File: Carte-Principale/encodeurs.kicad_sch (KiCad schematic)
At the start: 0 parts

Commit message: Moteurs + Encodeurs
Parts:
- added J3: Encodeur_G, symbol Connector:Conn_01x08_Pin
- added J4: Encodeur_D, symbol Connector:Conn_01x08_Pin
- added R1, R2, R3, R4: 100, symbol Device:R_Small
- added U6: AM26LV32xD, Package_SO:SOIC-16_3.9x9.9mm_P1.27mm, symbol Interface:AM26LV32xD
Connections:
- new net +3.3V: U6.16 (VDD), U6.4 (G)
- new net +5V: J3.1 (Pin_1), J4.1 (Pin_1)
- new net A+_DROITE: J4.6 (Pin_6), R4.2, U6.2 (1A)
- new net A+_GAUCHE: J3.6 (Pin_6), R2.2, U6.10 (3A)
- new net A-_DROITE: J4.7 (Pin_7), R4.1, U6.1 (1B)
- new net A-_GAUCHE: J3.7 (Pin_7), R2.1, U6.9 (3B)
- new net A_DROITE: U6.3 (1Y)
- new net A_GAUCHE: U6.11 (3Y)
- new net B+_DROITE: J4.5 (Pin_5), R3.2, U6.6 (2A)
- new net B+_GAUCHE: J3.5 (Pin_5), R1.2, U6.14 (4A)
- new net B-_DROITE: J4.4 (Pin_4), R3.1, U6.7 (2B)
- new net B-_GAUCHE: J3.4 (Pin_4), R1.1, U6.15 (4B)
- new net B_DROITE: U6.5 (2Y)
- new net B_GAUCHE: U6.13 (4Y)
- new net GND: J3.8 (Pin_8), J4.8 (Pin_8), U6.12 (~{G}), U6.8 (GND)
- new net Z+_DROITE: J4.2 (Pin_2)
- new net Z+_GAUCHE: J3.2 (Pin_2)
- new net Z-_DROITE: J4.3 (Pin_3)
- new net Z-_GAUCHE: J3.3 (Pin_3)
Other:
- note added: "Bien mettre dans le bon sens dans le PCB"

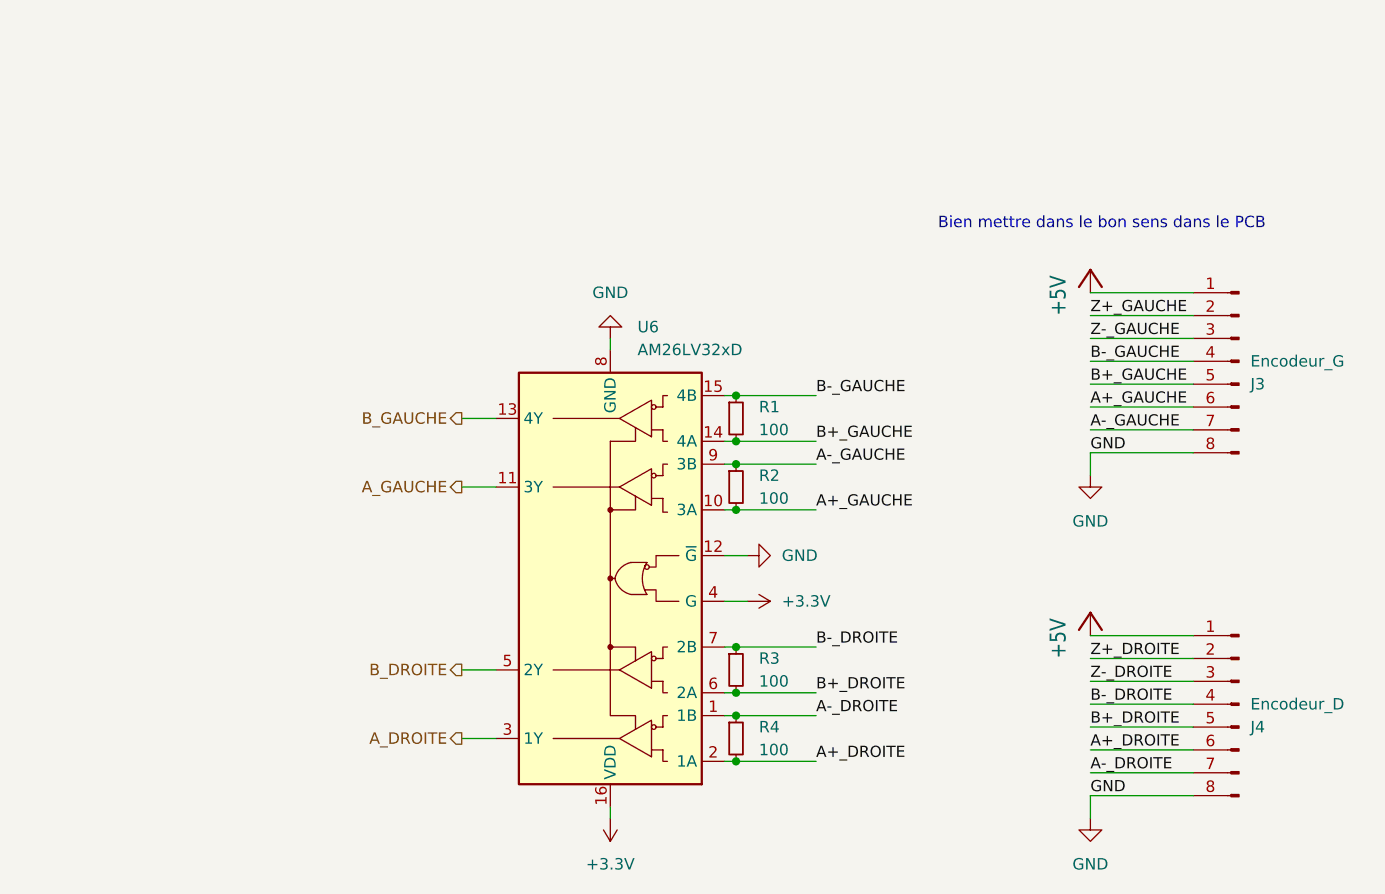
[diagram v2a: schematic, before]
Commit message: wiring
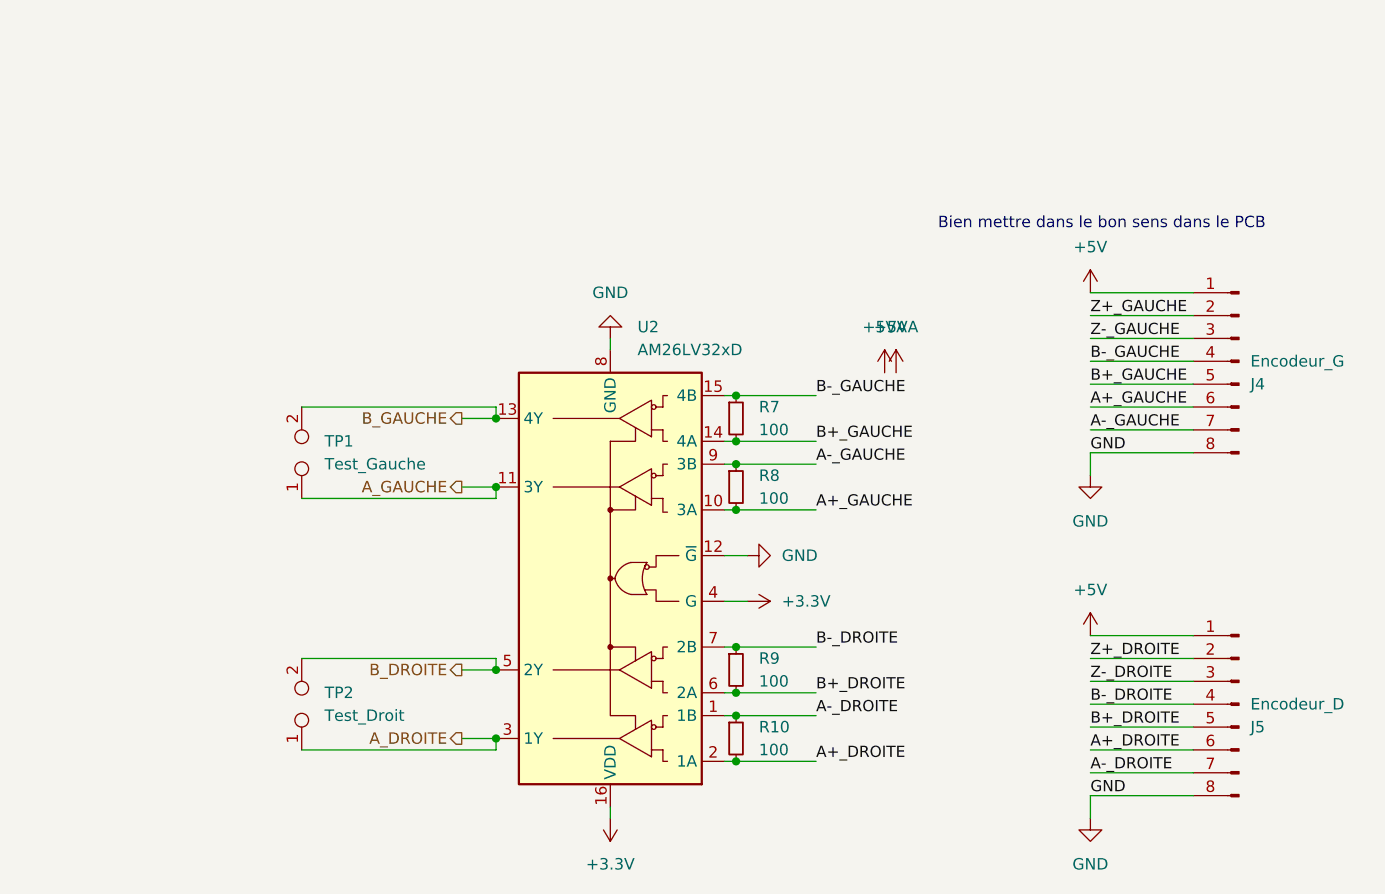
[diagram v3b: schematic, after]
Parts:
- added TP1: Test_Gauche, TestPoint:TestPoint_2Pads_Pitch2.54mm_Drill0.8mm, symbol Connector:TestPoint_2Pole
- added TP2: Test_Droit, TestPoint:TestPoint_2Pads_Pitch2.54mm_Drill0.8mm, symbol Connector:TestPoint_2Pole
- J4: renamed from J3; footprint (none) -> Connector_PinHeader_2.54mm:PinHeader_1x08_P2.54mm_Vertical
- J5: renamed from J4; footprint (none) -> Connector_PinHeader_2.54mm:PinHeader_1x08_P2.54mm_Vertical
- R10: renamed from R4; footprint (none) -> Resistor_THT:R_Axial_DIN0207_L6.3mm_D2.5mm_P10.16mm_Horizontal
- R7: renamed from R1; footprint (none) -> Resistor_THT:R_Axial_DIN0207_L6.3mm_D2.5mm_P10.16mm_Horizontal
- R8: renamed from R2; footprint (none) -> Resistor_THT:R_Axial_DIN0207_L6.3mm_D2.5mm_P10.16mm_Horizontal
- R9: renamed from R3; footprint (none) -> Resistor_THT:R_Axial_DIN0207_L6.3mm_D2.5mm_P10.16mm_Horizontal
- renumbered U6 to U2
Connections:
- net A_DROITE: now also TP2.1
- net A_GAUCHE: now also TP1.1
- net B_DROITE: now also TP2.2
- net B_GAUCHE: now also TP1.2

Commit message: Schéma vérifié
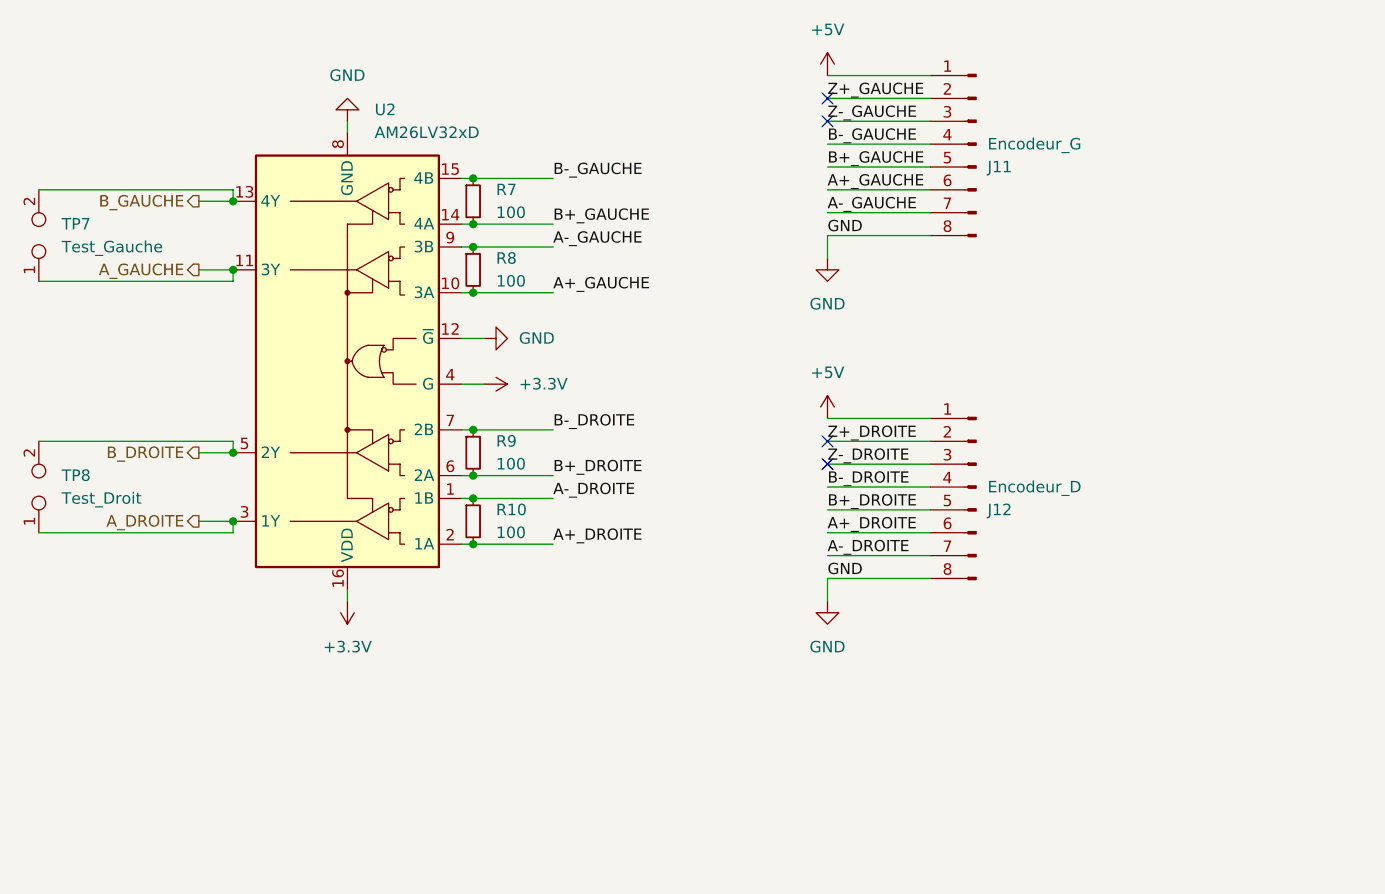
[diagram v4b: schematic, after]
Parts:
- renumbered J4 to J11, J5 to J12, TP1 to TP7, TP2 to TP8
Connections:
- no-connect marks 0 -> 4
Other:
- note removed: "Bien mettre dans le bon sens dans le PCB"
- company: (none) -> CRINSA
- title: (none) -> Carte Principale
- moved on the sheet: J11, J12, R10, R7, R8, R9, TP7, TP8, U2

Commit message: Avancée PCB
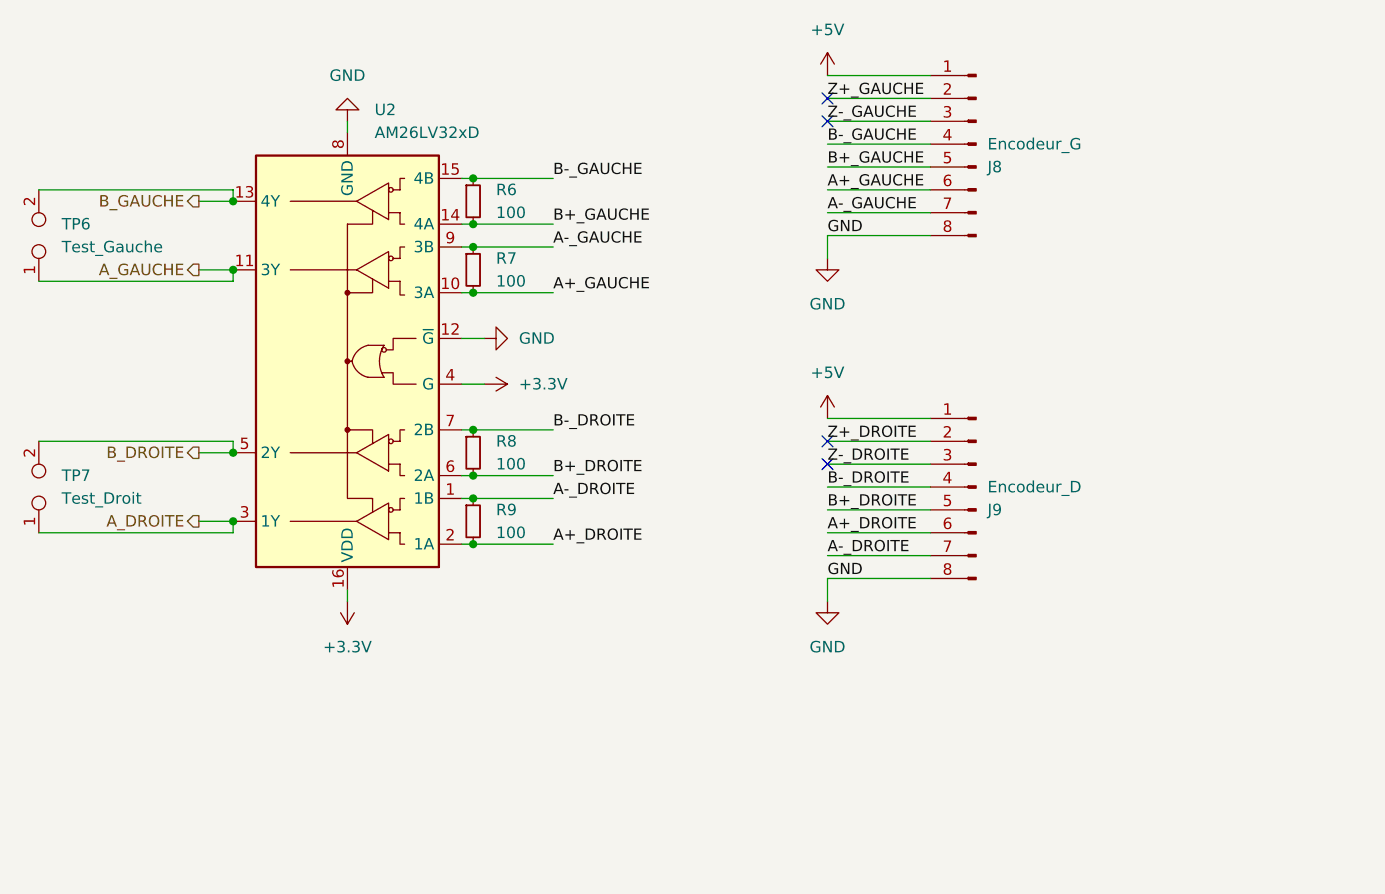
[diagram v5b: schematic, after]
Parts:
- J8: renamed from J11; footprint Connector_PinHeader_2.54mm:PinHeader_1x08_P2.54mm_Vertical -> Connector_Molex:Molex_KK-254_AE-6410-08A_1x08_P2.54mm_Vertical
- J9: renamed from J12; footprint Connector_PinHeader_2.54mm:PinHeader_1x08_P2.54mm_Vertical -> Connector_Molex:Molex_KK-254_AE-6410-08A_1x08_P2.54mm_Vertical
- R6: renamed from R7; footprint Resistor_THT:R_Axial_DIN0207_L6.3mm_D2.5mm_P10.16mm_Horizontal -> Resistor_SMD:R_1210_3225Metric_Pad1.30x2.65mm_HandSolder
- R7: renamed from R8; footprint Resistor_THT:R_Axial_DIN0207_L6.3mm_D2.5mm_P10.16mm_Horizontal -> Resistor_SMD:R_1210_3225Metric_Pad1.30x2.65mm_HandSolder
- R8: renamed from R9; footprint Resistor_THT:R_Axial_DIN0207_L6.3mm_D2.5mm_P10.16mm_Horizontal -> Resistor_SMD:R_1210_3225Metric_Pad1.30x2.65mm_HandSolder
- R9: renamed from R10; footprint Resistor_THT:R_Axial_DIN0207_L6.3mm_D2.5mm_P10.16mm_Horizontal -> Resistor_SMD:R_1210_3225Metric_Pad1.30x2.65mm_HandSolder
- renumbered TP7 to TP6, TP8 to TP7
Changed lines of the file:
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@@
 		(dnp no)
 		(fields_autoplaced yes)
-		(property "Reference" "#PWR040"
+		(property "Reference" "#PWR034"
 			(at 125.73 97.79 0)
 			(effects
@@
 			(project "Carte-Principale"
 				(path "/88b0dd29-ac24-4c5d-804c-fc642ecf6263/a2923913-7939-4f75-8694-93f1ab74a018"
-					(reference "#PWR040")
+					(reference "#PWR034")
 					(unit 1)
 				)
@@
 		(dnp no)
 		(fields_autoplaced yes)
-		(property "Reference" "TP8"
+		(property "Reference" "TP7"
 			(at 40.64 77.4699 90)
 			(effects
@@
 			(project "Carte-Principale"
 				(path "/88b0dd29-ac24-4c5d-804c-fc642ecf6263/a2923913-7939-4f75-8694-93f1ab74a018"
-					(reference "TP8")
+					(reference "TP7")
 					(unit 1)
 				)
@@
 		(dnp no)
 		(fields_autoplaced yes)
-		(property "Reference" "#PWR033"
+		(property "Reference" "#PWR027"
 			(at 125.73 36.83 0)
 			(effects
@@
 			(project "Carte-Principale"
 				(path "/88b0dd29-ac24-4c5d-804c-fc642ecf6263/a2923913-7939-4f75-8694-93f1ab74a018"
-					(reference "#PWR033")
+					(reference "#PWR027")
 					(unit 1)
 				)
@@
 		(dnp no)
 		(fields_autoplaced yes)
-		(property "Reference" "J12"
+		(property "Reference" "J9"
 			(at 143.51 81.2801 0)
 			(effects
@@
 			)
 		)
-		(property "Footprint" "Connector_PinHeader_2.54mm:PinHeader_1x08_P2.54mm_Vertical"
+		(property "Footprint" "Connector_Molex:Molex_KK-254_AE-6410-08A_1x08_P2.54mm_Vertical"
 			(at 142.24 78.74 0)
 			(effects
@@
 			(project "Carte-Principale"
 				(path "/88b0dd29-ac24-4c5d-804c-fc642ecf6263/a2923913-7939-4f75-8694-93f1ab74a018"
-					(reference "J12")
+					(reference "J9")
 					(unit 1)
 				)
@@
 		(dnp no)
 		(fields_autoplaced yes)
-		(property "Reference" "TP7"
+		(property "Reference" "TP6"
 			(at 40.64 49.5299 90)
 			(effects
@@
 			(project "Carte-Principale"
 				(path "/88b0dd29-ac24-4c5d-804c-fc642ecf6263/a2923913-7939-4f75-8694-93f1ab74a018"
-					(reference "TP7")
+					(reference "TP6")
 					(unit 1)
 				)
@@
 		(dnp no)
 		(fields_autoplaced yes)
-		(property "Reference" "#PWR038"
+		(property "Reference" "#PWR032"
 			(at 125.73 74.93 0)
 			(effects
@@
 			(project "Carte-Principale"
 				(path "/88b0dd29-ac24-4c5d-804c-fc642ecf6263/a2923913-7939-4f75-8694-93f1ab74a018"
-					(reference "#PWR038")
+					(reference "#PWR032")
 					(unit 1)
 				)
@@
 		(dnp no)
 		(fields_autoplaced yes)
-		(property "Reference" "R9"
+		(property "Reference" "R8"
 			(at 88.9 73.6599 0)
 			(effects
@@
 			)
 		)
-		(property "Footprint" "Resistor_THT:R_Axial_DIN0207_L6.3mm_D2.5mm_P10.16mm_Horizontal"
+		(property "Footprint" "Resistor_SMD:R_1210_3225Metric_Pad1.30x2.65mm_HandSolder"
 			(at 86.36 74.93 0)
 			(effects
@@
 			(project "Carte-Principale"
 				(path "/88b0dd29-ac24-4c5d-804c-fc642ecf6263/a2923913-7939-4f75-8694-93f1ab74a018"
-					(reference "R9")
+					(reference "R8")
 					(unit 1)
 				)
@@
 		(dnp no)
 		(fields_autoplaced yes)
-		(property "Reference" "R8"
+		(property "Reference" "R7"
 			(at 88.9 53.3399 0)
 			(effects
@@
 			)
 		)
-		(property "Footprint" "Resistor_THT:R_Axial_DIN0207_L6.3mm_D2.5mm_P10.16mm_Horizontal"
+		(property "Footprint" "Resistor_SMD:R_1210_3225Metric_Pad1.30x2.65mm_HandSolder"
 			(at 86.36 54.61 0)
 			(effects
@@
 			(project "Carte-Principale"
 				(path "/88b0dd29-ac24-4c5d-804c-fc642ecf6263/a2923913-7939-4f75-8694-93f1ab74a018"
-					(reference "R8")
+					(reference "R7")
 					(unit 1)
 				)
@@
 		(on_board yes)
 		(dnp no)
-		(property "Reference" "#PWR036"
+		(property "Reference" "#PWR030"
 			(at 93.98 62.23 0)
 			(effects
@@
 			(project "Carte-Principale"
 				(path "/88b0dd29-ac24-4c5d-804c-fc642ecf6263/a2923913-7939-4f75-8694-93f1ab74a018"
-					(reference "#PWR036")
+					(reference "#PWR030")
 					(unit 1)
 				)
@@
 		(dnp no)
 		(fields_autoplaced yes)
-		(property "Reference" "#PWR034"
+		(property "Reference" "#PWR028"
 			(at 72.39 31.75 0)
 			(effects
@@
 			(project "Carte-Principale"
 				(path "/88b0dd29-ac24-4c5d-804c-fc642ecf6263/a2923913-7939-4f75-8694-93f1ab74a018"
-					(reference "#PWR034")
+					(reference "#PWR028")
 					(unit 1)
 				)
@@
 		(dnp no)
 		(fields_autoplaced yes)
-		(property "Reference" "J11"
+		(property "Reference" "J8"
 			(at 143.51 43.1801 0)
 			(effects
@@
 			)
 		)
-		(property "Footprint" "Connector_PinHeader_2.54mm:PinHeader_1x08_P2.54mm_Vertical"
+		(property "Footprint" "Connector_Molex:Molex_KK-254_AE-6410-08A_1x08_P2.54mm_Vertical"
 			(at 142.24 40.64 0)
 			(effects
@@
 			(project "Carte-Principale"
 				(path "/88b0dd29-ac24-4c5d-804c-fc642ecf6263/a2923913-7939-4f75-8694-93f1ab74a018"
-					(reference "J11")
+					(reference "J8")
 					(unit 1)
 				)
@@
 		(dnp no)
 		(fields_autoplaced yes)
-		(property "Reference" "R7"
+		(property "Reference" "R6"
 			(at 88.9 45.7199 0)
 			(effects
@@
 			)
 		)
-		(property "Footprint" "Resistor_THT:R_Axial_DIN0207_L6.3mm_D2.5mm_P10.16mm_Horizontal"
+		(property "Footprint" "Resistor_SMD:R_1210_3225Metric_Pad1.30x2.65mm_HandSolder"
 			(at 86.36 46.99 0)
 			(effects
@@
 			(project "Carte-Principale"
 				(path "/88b0dd29-ac24-4c5d-804c-fc642ecf6263/a2923913-7939-4f75-8694-93f1ab74a018"
-					(reference "R7")
+					(reference "R6")
 					(unit 1)
 				)
@@
 		(on_board yes)
 		(dnp no)
-		(property "Reference" "#PWR037"
+		(property "Reference" "#PWR031"
 			(at 83.82 67.31 0)
 			(effects
@@
 			(project "Carte-Principale"
 				(path "/88b0dd29-ac24-4c5d-804c-fc642ecf6263/a2923913-7939-4f75-8694-93f1ab74a018"
-					(reference "#PWR037")
+					(reference "#PWR031")
 					(unit 1)
 				)
@@
 		(dnp no)
 		(fields_autoplaced yes)
-		(property "Reference" "#PWR039"
+		(property "Reference" "#PWR033"
 			(at 72.39 87.63 0)
 			(effects
@@
 			(project "Carte-Principale"
 				(path "/88b0dd29-ac24-4c5d-804c-fc642ecf6263/a2923913-7939-4f75-8694-93f1ab74a018"
-					(reference "#PWR039")
+					(reference "#PWR033")
 					(unit 1)
 				)
@@
 		(dnp no)
 		(fields_autoplaced yes)
-		(property "Reference" "R10"
+		(property "Reference" "R9"
 			(at 88.9 81.2799 0)
 			(effects
@@
 			)
 		)
-		(property "Footprint" "Resistor_THT:R_Axial_DIN0207_L6.3mm_D2.5mm_P10.16mm_Horizontal"
+		(property "Footprint" "Resistor_SMD:R_1210_3225Metric_Pad1.30x2.65mm_HandSolder"
 			(at 86.36 82.55 0)
 			(effects
@@
 			(project "Carte-Principale"
 				(path "/88b0dd29-ac24-4c5d-804c-fc642ecf6263/a2923913-7939-4f75-8694-93f1ab74a018"
-					(reference "R10")
+					(reference "R9")
 					(unit 1)
 				)
@@
 		(dnp no)
 		(fields_autoplaced yes)
-		(property "Reference" "#PWR035"
+		(property "Reference" "#PWR029"
 			(at 125.73 59.69 0)
 			(effects
@@
 			(project "Carte-Principale"
 				(path "/88b0dd29-ac24-4c5d-804c-fc642ecf6263/a2923913-7939-4f75-8694-93f1ab74a018"
-					(reference "#PWR035")
-					(unit 1)
-				)
+					(reference "#PWR029")
+					(unit 1)
+				)
